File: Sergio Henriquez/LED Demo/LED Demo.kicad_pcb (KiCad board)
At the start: 2 copper layers, 15 x 11 mm, 3 parts

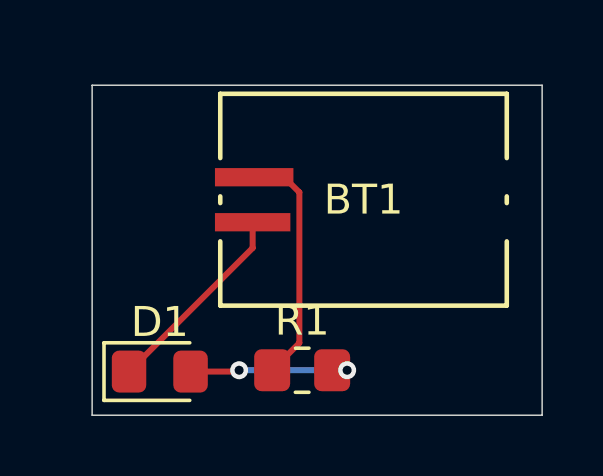
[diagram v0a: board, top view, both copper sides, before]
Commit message: LED demo
kicad intro
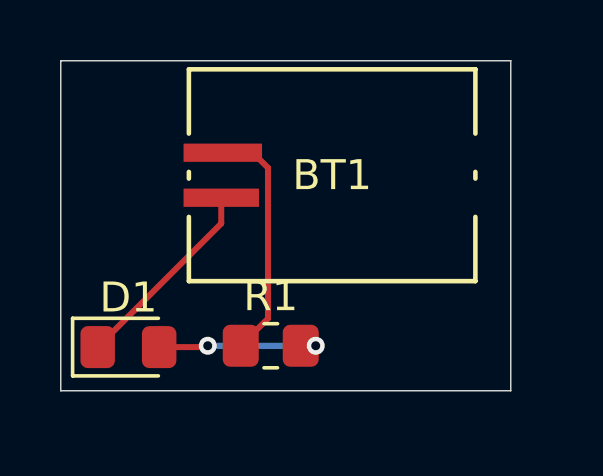
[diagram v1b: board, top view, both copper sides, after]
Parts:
- moved R1 1.33 mm to (126.0, 83.2)
- moved BT1 1.33 mm to (128.0, 77.5)
- moved D1 1.33 mm to (121.2, 83.2)
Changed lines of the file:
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@@
 	(footprint "Resistor_SMD:R_0805_2012Metric_Pad1.20x1.40mm_HandSolder"
 		(layer "F.Cu")
-		(at 127 84)
+		(at 125.953796 83.183796)
 		(descr "Resistor SMD 0805 (2012 Metric), square (rectangular) end terminal, IPC_7351 nominal with elongated pad for handsoldering. (Body size source: IPC-SM-782 page 72, https://www.pcb-3d.com/wordpress/wp-content/uploads/ipc-sm-782a_amendment_1_and_2.pdf), generated with kicad-footprint-generator")
 		(tags "resistor handsolder")
@@
 	(footprint "FS_3_Global_Footprint_Library:MS621FE-FL11E_SEC"
 		(layer "F.Cu")
-		(at 129.046204 78.316204)
+		(at 128 77.5)
 		(descr "Coin Cell Battery")
 		(tags "MS621FE-FL11E ")
@@
 	(footprint "LED_SMD:LED_0805_2012Metric_Pad1.15x1.40mm_HandSolder"
 		(layer "F.Cu")
-		(at 122.255 84.045)
+		(at 121.208796 83.228796)
 		(descr "LED SMD 0805 (2012 Metric), square (rectangular) end terminal, IPC_7351 nominal, (Body size source: https://docs.google.com/spreadsheets/d/1BsfQQcO9C6DZCsRaXUlFlo91Tg2WpOkGARC1WS5S8t0/edit?usp=sharing), generated with kicad-footprint-generator")
 		(tags "LED handsolder")
@@
 	)
 	(gr_rect
-		(start 120 74.5)
-		(end 135 85.5)
+		(start 118.953796 73.683796)
+		(end 133.953796 84.683796)
 		(stroke
 			(width 0.05)
@@
 	)
 	(segment
-		(start 125.350504 79.066205)
-		(end 125.350504 79.924496)
+		(start 124.3043 78.250001)
+		(end 124.3043 79.108292)
 		(width 0.2)
 		(layer "F.Cu")
@@
 	)
 	(segment
-		(start 125.350504 79.924496)
-		(end 121.23 84.045)
+		(start 124.3043 79.108292)
+		(end 120.183796 83.228796)
 		(width 0.2)
 		(layer "F.Cu")
@@
 	)
 	(segment
-		(start 126.907804 78.069403)
-		(end 126.907804 83.092196)
+		(start 125.8616 77.253199)
+		(end 125.8616 82.275992)
 		(width 0.2)
 		(layer "F.Cu")
@@
 	)
 	(segment
-		(start 126.404604 77.566203)
-		(end 126.907804 78.069403)
+		(start 125.3584 76.749999)
+		(end 125.8616 77.253199)
 		(width 0.2)
 		(layer "F.Cu")
@@
 	)
 	(segment
-		(start 126.907804 83.092196)
-		(end 126 84)
+		(start 125.8616 82.275992)
+		(end 124.953796 83.183796)
 		(width 0.2)
 		(layer "F.Cu")
@@
 	)
 	(segment
-		(start 125.401304 77.566203)
-		(end 126.404604 77.566203)
+		(start 124.3551 76.749999)
+		(end 125.3584 76.749999)
 		(width 0.2)
 		(layer "F.Cu")
@@
 	)
 	(segment
-		(start 124.855 84.045)
-		(end 124.9 84)
+		(start 123.808796 83.228796)
+		(end 123.853796 83.183796)
 		(width 0.2)
 		(layer "F.Cu")
@@
 	)
 	(segment
-		(start 123.28 84.045)
-		(end 124.855 84.045)
+		(start 122.233796 83.228796)
+		(end 123.808796 83.228796)
 		(width 0.2)
 		(layer "F.Cu")
@@
 	)
 	(via
-		(at 128.5 84)
+		(at 127.453796 83.183796)
 		(size 0.6)
 		(drill 0.3)
@@
 	)
 	(via
-		(at 124.9 84)
+		(at 123.853796 83.183796)
 		(size 0.6)
 		(drill 0.3)
@@
 	)
 	(segment
-		(start 124.9 84)
-		(end 128.5 84)
+		(start 123.853796 83.183796)
+		(end 127.453796 83.183796)
 		(width 0.2)
 		(layer "B.Cu")
